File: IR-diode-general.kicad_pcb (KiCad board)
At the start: 2 copper layers, 80 x 20.5 mm, 39 parts, among them J1 BarrelJack_3167288, J2 USB4105-GF-A, U1 QFN10_MP2483DQ_MNP, U2 AP62301Z6-7, U3 SM02B-SRSS-TB-LF-SN, U4 SM02B-SRSS-TB-LF-SN

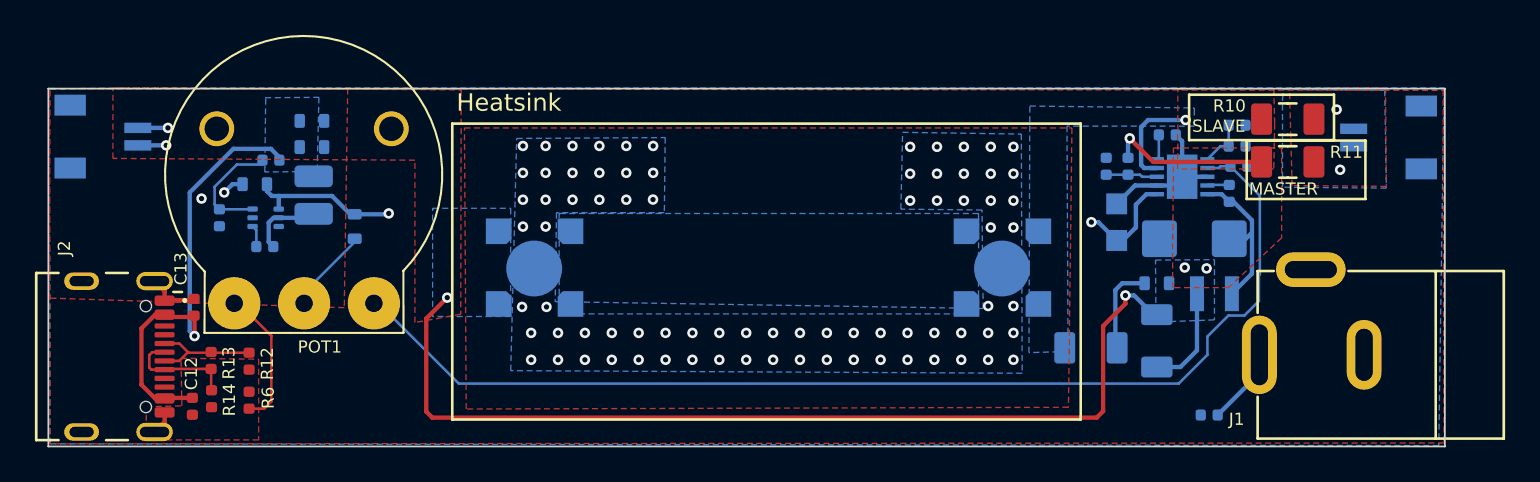
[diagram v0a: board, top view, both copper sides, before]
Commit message: Added signage
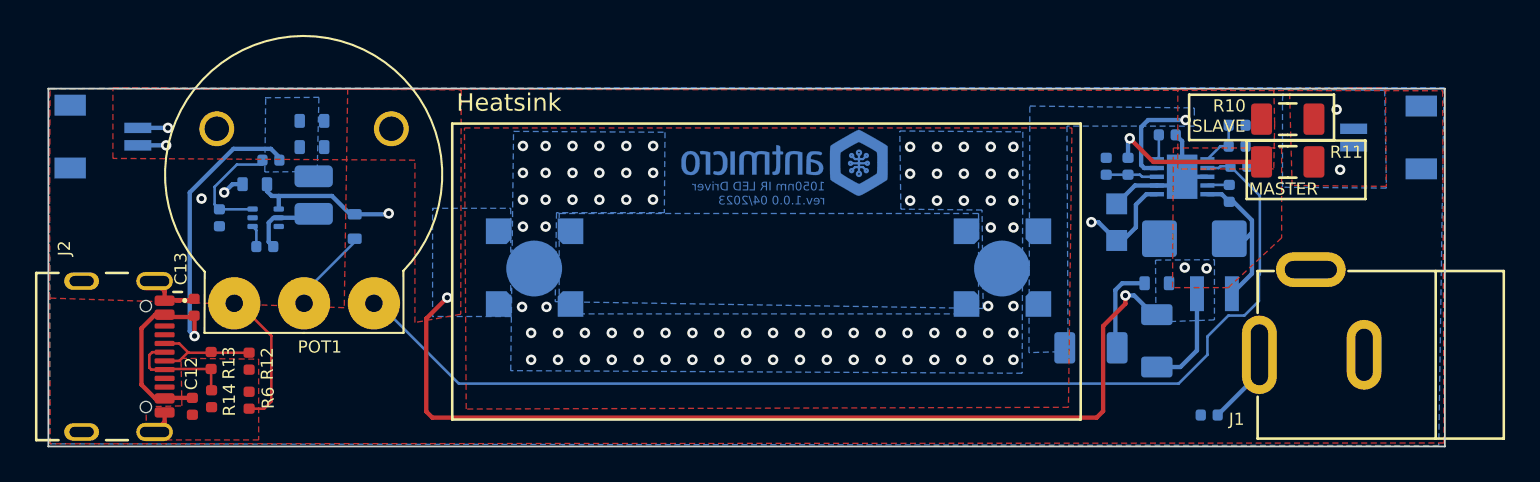
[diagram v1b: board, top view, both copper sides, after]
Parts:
- added N1: antmicro_logo, antmicro-footprints:antmicro-logo_scaled_12mm, B.Cu at (127.2, 44.8)
- U1: value QFN10_MP2483DQ_MNP -> MP2483DQ-LF-P
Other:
- board text added: "1050nm IR LED Driver rev.1.0.0 04/2023"
